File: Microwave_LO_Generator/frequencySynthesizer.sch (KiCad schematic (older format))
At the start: 29 parts, among them J1 BNC_THT, J2 SMA_END, J3 SMA_END, U1 ADF4150HV, X1 IQXT-220-1

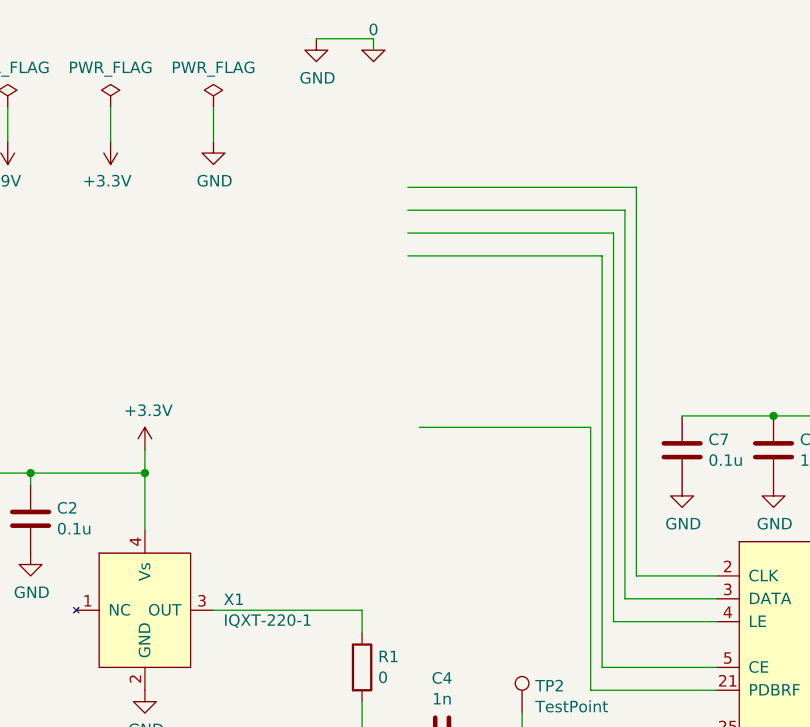
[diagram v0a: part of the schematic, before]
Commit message: Update
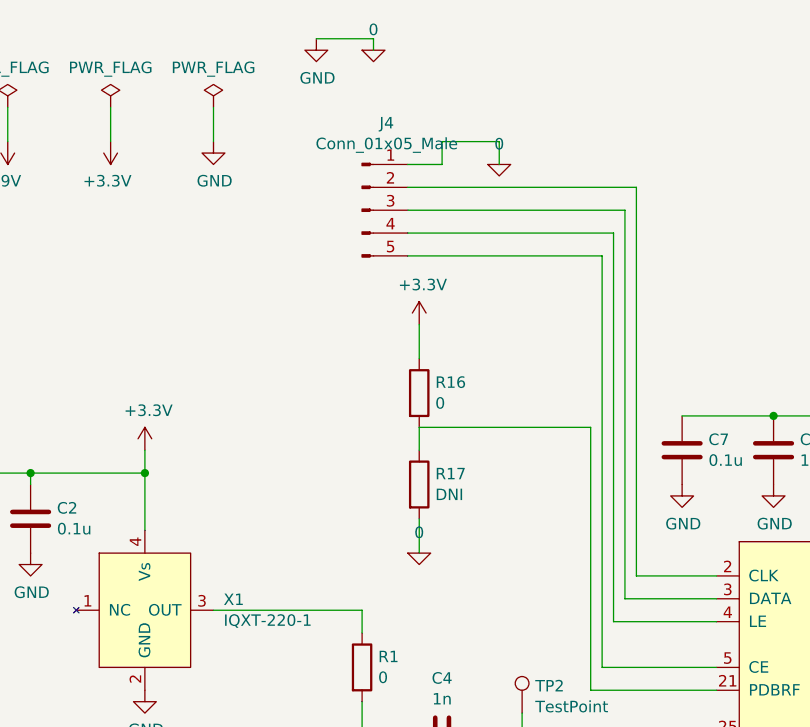
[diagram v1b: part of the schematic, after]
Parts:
- added J4: Conn_01x05_Male, Connector_PinHeader_2.54mm:PinHeader_1x05_P2.54mm_Vertical, symbol Connector:Conn_01x05_Male
- added R16: 0, Resistor_SMD:R_0402_1005Metric_Pad0.72x0.64mm_HandSolder, symbol Device:R
- added R17: DNI, Resistor_SMD:R_0603_1608Metric_Pad0.98x0.95mm_HandSolder, symbol Device:R
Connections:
- wire segments 88 -> 95
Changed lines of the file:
@@
 	2500 1350 2500 1500
-$Comp
-L power:+3.3V #PWR0103
-U 1 1 5FB52FA7
-P 5250 2550
-F 0 "#PWR0103" H 5250 2400 50  0001 C CNN
-F 1 "+3.3V" H 5265 2723 50  0000 C CNN
-F 2 "" H 5250 2550 50  0001 C CNN
-F 3 "" H 5250 2550 50  0001 C CNN
-	1    5250 2550
-	1    0    0    -1
-$EndComp
 $Comp
 L power:+9V #PWR0104
@@
 	5450 2450 5450 2700
 Wire Wire Line
-	5250 2550 5250 2700
-Wire Wire Line
 	5350 2700 5450 2700
 Connection ~ 5450 2700
@@
 	1    0    0    -1
 $EndComp
-Connection ~ 5250 2700
 Wire Wire Line
 	5250 2700 5250 3150
@@
 Wire Wire Line
 	3200 1050 3200 1100
+$Comp
+L pspice:0 #GND0122
+U 1 1 5FCD8892
+P 3750 1600
+F 0 "#GND0122" H 3750 1500 50  0001 C CNN
+F 1 "0" H 3750 1689 50  0000 C CNN
+F 2 "" H 3750 1600 50  0001 C CNN
+F 3 "~" H 3750 1600 50  0001 C CNN
+	1    3750 1600
+	1    0    0    -1
+$EndComp
+Wire Wire Line
+	3750 1500 3750 1600
+$Comp
+L Connector:Conn_01x05_Male J4
+U 1 1 5FCD328E
+P 3150 1800
+F 0 "J4" H 3258 2181 50  0000 C CNN
+F 1 "Conn_01x05_Male" H 3258 2090 50  0000 C CNN
+F 2 "Connector_PinHeader_2.54mm:PinHeader_1x05_P2.54mm_Vertical" H 3150 1800 50  0001 C CNN
+F 3 "~" H 3150 1800 50  0001 C CNN
+	1    3150 1800
+	1    0    0    -1
+$EndComp
+Wire Wire Line
+	3500 1500 3500 1600
+Wire Wire Line
+	3500 1600 3350 1600
+Wire Wire Line
+	3500 1500 3750 1500
+$Comp
+L Device:R R17
+U 1 1 5FD3B0E5
+P 3400 3000
+F 0 "R17" H 3470 3046 50  0000 L CNN
+F 1 "DNI" H 3470 2955 50  0000 L CNN
+F 2 "Resistor_SMD:R_0603_1608Metric_Pad0.98x0.95mm_HandSolder" V 3330 3000 50  0001 C CNN
+F 3 "~" H 3400 3000 50  0001 C CNN
+F 4 "D/CRCW0402 kit in dipartimento" H 3400 3000 50  0001 C CNN "Supplier Stock Code"
+	1    3400 3000
+	1    0    0    -1
+$EndComp
+Wire Wire Line
+	3400 3150 3400 3300
+Wire Wire Line
+	3400 2750 3400 2850
+$Comp
+L Device:R R16
+U 1 1 5FD46A04
+P 3400 2600
+F 0 "R16" H 3470 2646 50  0000 L CNN
+F 1 "0" H 3470 2555 50  0000 L CNN
+F 2 "Resistor_SMD:R_0402_1005Metric_Pad0.72x0.64mm_HandSolder" V 3330 2600 50  0001 C CNN
+F 3 "~" H 3400 2600 50  0001 C CNN
+F 4 "D/CRCW0402 kit in dipartimento" H 3400 2600 50  0001 C CNN "Supplier Stock Code"
+	1    3400 2600
+	1    0    0    -1
+$EndComp
+$Comp
+L pspice:0 #GND0123
+U 1 1 5FD49CF4
+P 3400 3300
+F 0 "#GND0123" H 3400 3200 50  0001 C CNN
+F 1 "0" H 3400 3389 50  0000 C CNN
+F 2 "" H 3400 3300 50  0001 C CNN
+F 3 "~" H 3400 3300 50  0001 C CNN
+	1    3400 3300
+	1    0    0    -1
+$EndComp
+Connection ~ 5250 2700
+Wire Wire Line
+	5250 2550 5250 2700
+$Comp
+L power:+3.3V #PWR0103
+U 1 1 5FB52FA7
+P 5250 2550
+F 0 "#PWR0103" H 5250 2400 50  0001 C CNN
+F 1 "+3.3V" H 5265 2723 50  0000 C CNN
+F 2 "" H 5250 2550 50  0001 C CNN
+F 3 "" H 5250 2550 50  0001 C CNN
+	1    5250 2550
+	1    0    0    -1
+$EndComp
+$Comp
+L power:+3.3V #PWR0138
+U 1 1 5FD4CD79
+P 3400 2300
+F 0 "#PWR0138" H 3400 2150 50  0001 C CNN
+F 1 "+3.3V" H 3415 2473 50  0000 C CNN
+F 2 "" H 3400 2300 50  0001 C CNN
+F 3 "" H 3400 2300 50  0001 C CNN
+	1    3400 2300
+	1    0    0    -1
+$EndComp
+Wire Wire Line
+	3400 2300 3400 2450
 $EndSCHEMATC
